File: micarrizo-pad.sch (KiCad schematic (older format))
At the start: 20 parts, among them U1 The-Big-Switch, U2 KB2040

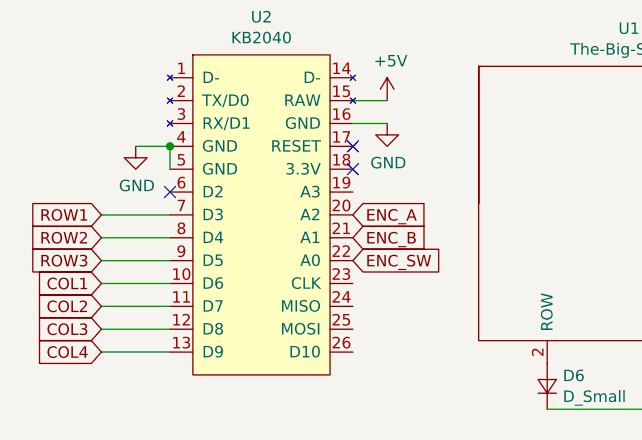
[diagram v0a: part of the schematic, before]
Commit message: finish pcb
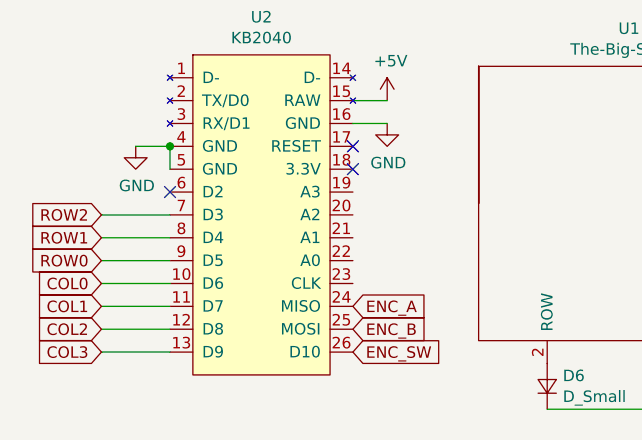
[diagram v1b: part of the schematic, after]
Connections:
- net COL4 is gone; now on net COL3: U2.13 (D9)
- net ROW3 is gone; now on net ROW0: U2.9 (D5)
- net COL0: now also U2.10 (D6)
- net COL1: now also U2.11 (D7); no longer U2.10 (D6)
- net COL2: now also U2.12 (D8); no longer U2.11 (D7)
- net COL3: no longer U2.12 (D8)
- net ENC_A: now also U2.24 (MISO); no longer U2.20 (A2)
- net ENC_B: now also U2.25 (MOSI); no longer U2.21 (A1)
- net ENC_SW: now also U2.26 (D10); no longer U2.22 (A0)
- net ROW1: now also U2.8 (D4); no longer U2.7 (D3)
- net ROW2: now also U2.7 (D3); no longer U2.8 (D4)
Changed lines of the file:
@@
 Text GLabel 5500 2400 1    50   Input ~ 0
 COL0
+Text GLabel 2550 3850 0    50   Input ~ 0
+ROW0
+Text GLabel 2550 3750 0    50   Input ~ 0
+ROW1
 Text GLabel 2550 3650 0    50   Input ~ 0
-ROW1
-Text GLabel 2550 3750 0    50   Input ~ 0
 ROW2
-Text GLabel 2550 3850 0    50   Input ~ 0
-ROW3
 Text GLabel 2550 3950 0    50   Input ~ 0
+COL0
+Text GLabel 2550 4050 0    50   Input ~ 0
 COL1
-Text GLabel 2550 4050 0    50   Input ~ 0
+Text GLabel 2550 4150 0    50   Input ~ 0
 COL2
-Text GLabel 2550 4150 0    50   Input ~ 0
+Text GLabel 2550 4250 0    50   Input ~ 0
 COL3
-Text GLabel 2550 4250 0    50   Input ~ 0
-COL4
 Wire Wire Line
 	2550 3650 2850 3650
@@
 Text GLabel 8300 3750 0    50   Input ~ 0
 ENC_B
-Text GLabel 3650 3850 2    50   Input ~ 0
+Text GLabel 3650 4250 2    50   Input ~ 0
 ENC_SW
-Text GLabel 3650 3650 2    50   Input ~ 0
+Text GLabel 3650 4050 2    50   Input ~ 0
 ENC_A
-Text GLabel 3650 3750 2    50   Input ~ 0
+Text GLabel 3650 4150 2    50   Input ~ 0
 ENC_B
 $EndSCHEMATC
